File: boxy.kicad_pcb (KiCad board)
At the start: 2 copper layers, 31.5 x 35.6 mm, 25 parts, among them P1 Isolated interface, Q1 NPN, U1 TRIAC, U2 OPTO-TRANSISTOR, U3 OPTO-TRIAC

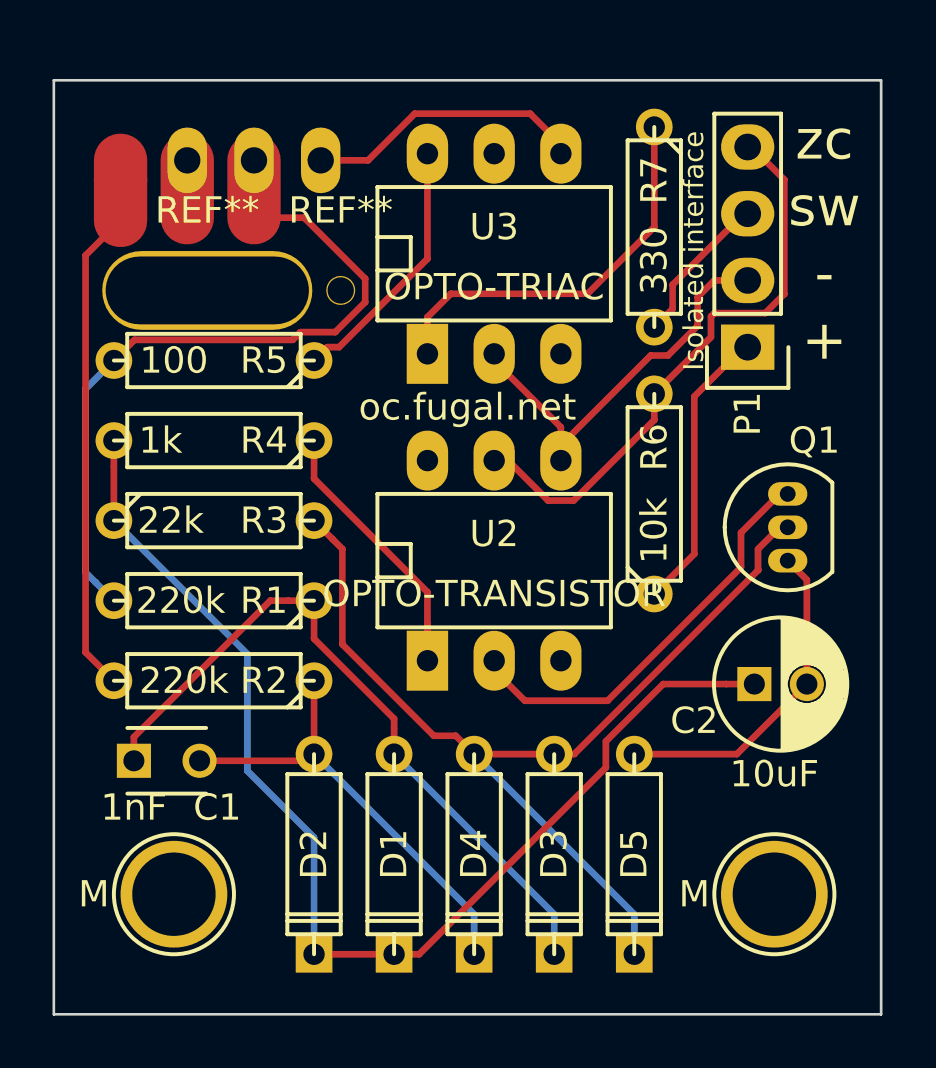
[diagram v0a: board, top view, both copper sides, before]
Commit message: boxy with smd resistors
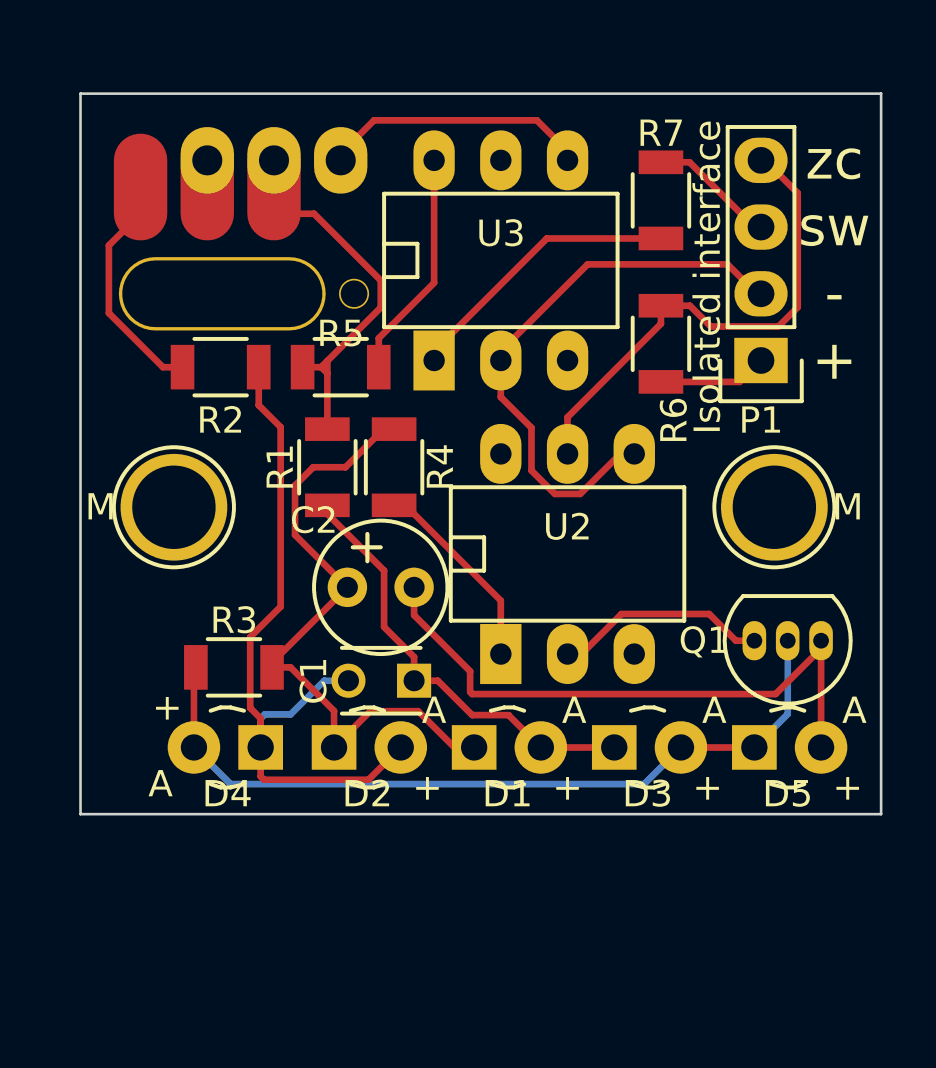
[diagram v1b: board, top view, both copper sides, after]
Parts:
- removed the REF** at (42.7, 53.8)
- removed the REF** at (34.5, 38.1)
- added ?: Symbol_OSHW-Logo_SilkScreen, Symbols:Symbol_OSHW-Logo_SilkScreen, B.Cu at (39.1, 37.6)
- C2: footprint Capacitors_ThroughHole:C_Radial_D5_L11_P2 -> Capacitors_Elko_ThroughHole:Elko_vert_11x5mm_RM2.5
- D1, D2, D3, D4, D5: footprint Discret:D3 -> Diodes_ThroughHole:Diode_LED_3mm_round_vertical
- Q1: value NPN -> Q_NPN_EBC
- R1, R2, R3, R4, R5, R6, R7: footprint Discret:R3 -> Resistors_SMD:R_1206
- U1: footprint Transistors_TO-220:TO-220_Neutral123_Vertical -> Power_Integrations:TO-220
- moved C2 15.9 mm to (39.6, 43.7)
- moved M 14.7 mm to (33.0, 40.6)
- moved M 14.7 mm to (55.9, 40.6)
- moved R2 11.9 mm to (34.8, 35.3)
- moved C1 11.1 mm to (42.2, 47.2), turned to 180 degrees
- moved D4 10.2 mm to (35.1, 49.8), turned to 0 degrees
- moved D5 7.12 mm to (56.4, 49.8), turned to 180 degrees
- moved R4 6.93 mm to (41.4, 39.1), turned to 90 degrees
- moved R1 6.67 mm to (38.9, 39.1), turned to 90 degrees
- moved D1 5.93 mm to (45.7, 49.8), turned to 180 degrees
- moved R6 5.72 mm to (51.6, 34.4)
- moved R3 5.64 mm to (35.3, 46.7), turned to 180 degrees
- moved D3 5.40 mm to (51.1, 49.8), turned to 180 degrees
- moved R5 4.83 mm to (39.4, 35.3)
- moved D2 4.54 mm to (40.4, 49.8), turned to 180 degrees
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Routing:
- net Net-(C2-Pad1): track 44.3 -> 24.5 mm
- net Hot: track 28.8 -> 15.0 mm
- net N: track 20.8 -> 9.97 mm
- net Net-(C1-Pad2): track 17.4 -> 28.0 mm
- net Net-(C1-Pad1): track 27.2 -> 16.7 mm
- net Net-(C2-Pad2): track 13.0 -> 23.3 mm
- net Net-(Q1-Pad3): track 16.0 -> 8.16 mm
- net Net-(D3-Pad1): track 38.1 -> 31.0 mm
- net Net-(P1-Pad1): track 11.0 -> 4.15 mm
- net Net-(P1-Pad2): track 16.4 -> 22.0 mm
- net Net-(R7-Pad1): track 15.3 -> 10.8 mm
- net Net-(P1-Pad4): track 22.2 -> 19.2 mm
- net Net-(R4-Pad1): track 10.2 -> 7.60 mm
- net Net-(R5-Pad1): track 9.92 -> 8.75 mm
- net Net-(P1-Pad3): track 5.88 -> 4.83 mm
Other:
- board size 31.5 x 35.6 mm -> 30.5 x 27.4 mm
- board text removed: "oc.fugal.net"
